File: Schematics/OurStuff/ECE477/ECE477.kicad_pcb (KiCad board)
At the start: 2 copper layers, 90 x 40.5 mm, 65 parts, among them J1 USB_B_Micro, J2 Barrel_Jack, J3 OLED JST PH 7pin, J7 D30V30F3, Q1 SS8050-G, Q2 SS8050-G, U1 ESP32-WROOM-32E, U2 CP2102N-Axx-xQFN28

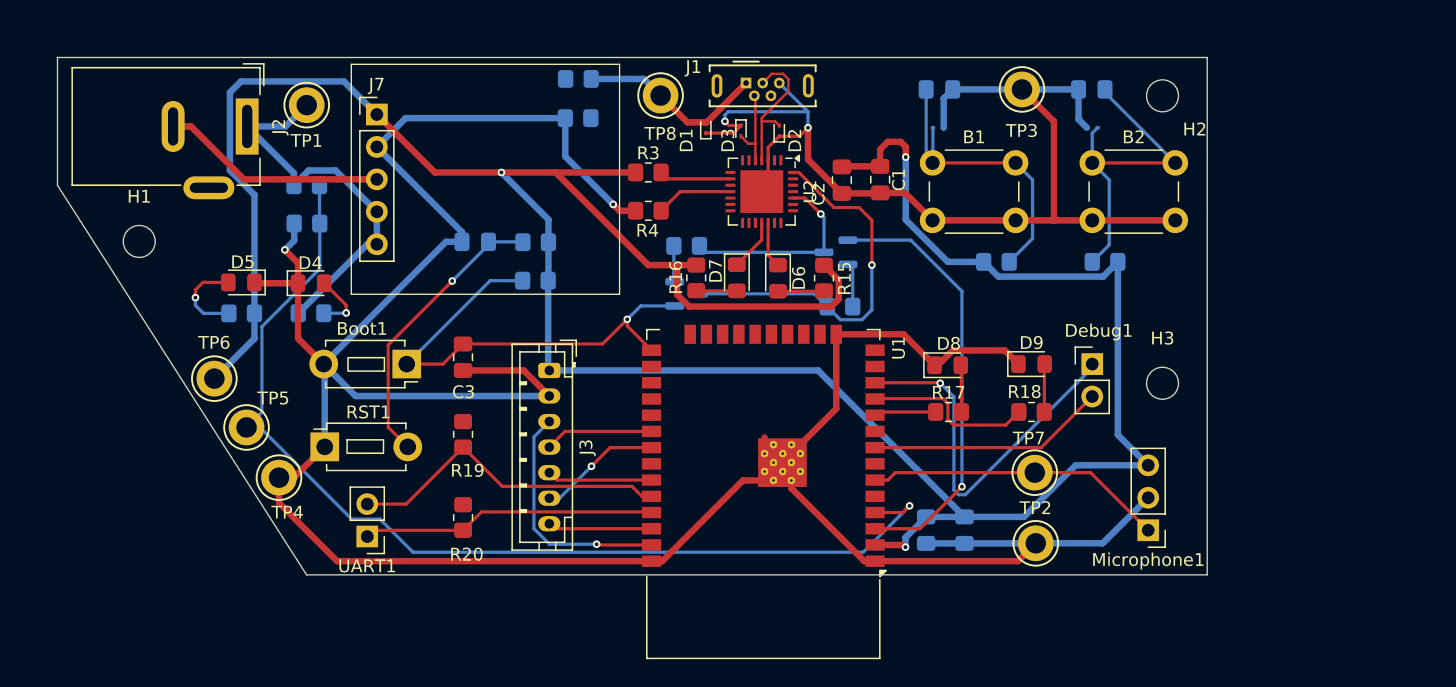
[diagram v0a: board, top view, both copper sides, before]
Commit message: hell yeah
pcb complete ver 1 (no more deletes please)
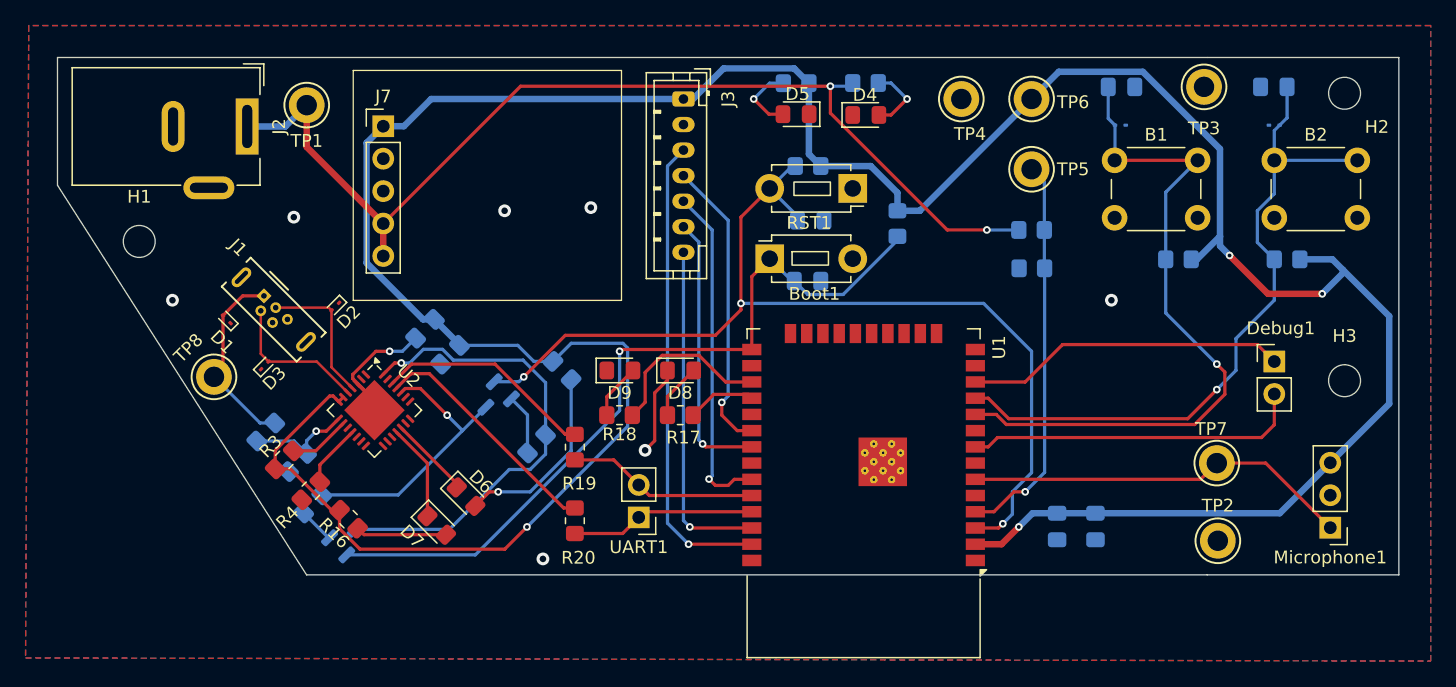
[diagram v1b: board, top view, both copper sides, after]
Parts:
- C1, C2, C3, R15: moved to B.Cu
- moved TP6 67.6 mm to (176.2, 53.2)
- moved TP5 64.7 mm to (176.2, 58.8)
- moved TP4 61.1 mm to (170.8, 53.2)
- moved R7 56.8 mm to (176.3, 66.5)
- moved R6 56.8 mm to (176.2, 63.5)
- moved R5 47.0 mm to (163.2, 52.0)
- moved R13 47.0 mm to (157.8, 52.0)
- moved RST1 46.0 mm to (162.2, 60.2), turned to 180 degrees
- moved D4 45.4 mm to (163.3, 54.5)
- moved D5 45.4 mm to (157.8, 54.4)
- moved D3 41.5 mm to (116.2, 74.1), turned to 45 degrees
- moved TP8 41.3 mm to (112.2, 75.0)
- moved J1 41.3 mm to (116.2, 68.7), turned to -45 degrees
- moved D1 40.4 mm to (113.2, 70.5), turned to 135 degrees
- moved C1 37.5 mm to (128.8, 71.2), turned to -135 degrees
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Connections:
- B1 pad 2: GND -> Gnd_Bat
- B2 pad 2: GND -> Gnd_Bat
- Boot1 pad 2: GND -> Gnd_Bat
- C1 pad 2: GND -> Gnd_Bat
- C2 pad 2: GND -> Gnd_Bat
- C3 pad 1: GND -> Gnd_Bat
- C4 pad 2: GND -> Gnd_Bat
- C6 pad 2: GND -> Gnd_Bat
- C7 pad 2: GND -> Gnd_Bat
- C8 pad 2: GND -> Gnd_Bat
- C9 pad 2: GND -> Gnd_Bat
- D1 pad 1: GND -> Gnd_Bat
- D10 pad 2: GND -> Gnd_Bat
- D11 pad 1: GND -> Gnd_Bat
- D2 pad 1: GND -> Gnd_Bat
- D3 pad 1: GND -> Gnd_Bat
- D4 pad 1: GND -> Gnd_Bat
- D5 pad 1: GND -> Gnd_Bat
- D8 pad 1: GND -> Gnd_Bat
- D9 pad 1: GND -> Gnd_Bat
- J1 pad 5: GND -> Gnd_Bat
- J3 pad 2: GND -> Gnd_Bat
- J7 pad 2: GND -> Gnd_Bat
- Microphone1 pad 2: GND -> Gnd_Bat
- R2 pad 2: GND -> Gnd_Bat
- R4 pad 1: GND -> Gnd_Bat
- R7 pad 2: GND -> Gnd_Bat
- RST1 pad 1: GND -> Gnd_Bat
- TP2 pad 1: GND -> Gnd_Bat
- TP3 pad 1: GND -> Gnd_Bat
- TP4 pad 1: GND -> Gnd_Bat
- U1 pad 1: GND -> Gnd_Bat
- U1 pad 10: /Debug_1 -> /Button1
- U1 pad 11: /Debug_2 -> /Button2
- U1 pad 15: GND -> Gnd_Bat
- U1 pad 27: /Button1 -> /Debug_2
- U1 pad 28: /Button2 -> /Debug_1
- U1 pad 38: GND -> Gnd_Bat
- U1 pad 39: GND -> Gnd_Bat
- U2 pad 29: GND -> Gnd_Bat
- U2 pad 3: GND -> Gnd_Bat
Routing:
- net GND: track 305.7 -> 0.00 mm, vias 4 -> 0
- net Vbat: track 30.7 -> 81.6 mm, vias 0 -> 2
- net BAT_ADC: track 81.7 -> 30.8 mm
- net /Button1: track 24.3 -> 54.6 mm, vias 0 -> 1
- net /Button2: track 26.3 -> 54.1 mm, vias 0 -> 1
- net +3.3V: track 219.6 -> 244.1 mm, vias 3 -> 4
- net /IO0: track 37.8 -> 62.0 mm
- net /EN: track 56.7 -> 79.2 mm, vias 2 -> 3
- net Net-(U2-RXD): track 0.00 -> 18.8 mm
- net /O_RST: track 8.16 -> 26.6 mm, vias 0 -> 1
- net /O_DIN: track 18.6 -> 37.0 mm
- net /O_CS: track 8.24 -> 26.5 mm, vias 0 -> 1
- net Net-(U2-TXD): track 0.00 -> 17.2 mm
- net /O_CLK: track 8.51 -> 23.3 mm, vias 0 -> 1
- net /O_DC: track 9.64 -> 21.6 mm
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- added copper zone on B.Cu, net Gnd_Bat
- added copper zone on F.Cu, net Gnd_Bat
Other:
- board size 90 x 40.5 mm -> 105 x 40.5 mm
